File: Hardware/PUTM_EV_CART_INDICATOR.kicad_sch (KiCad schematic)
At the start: 11 parts, among them J3 Screw_Terminal_01x06

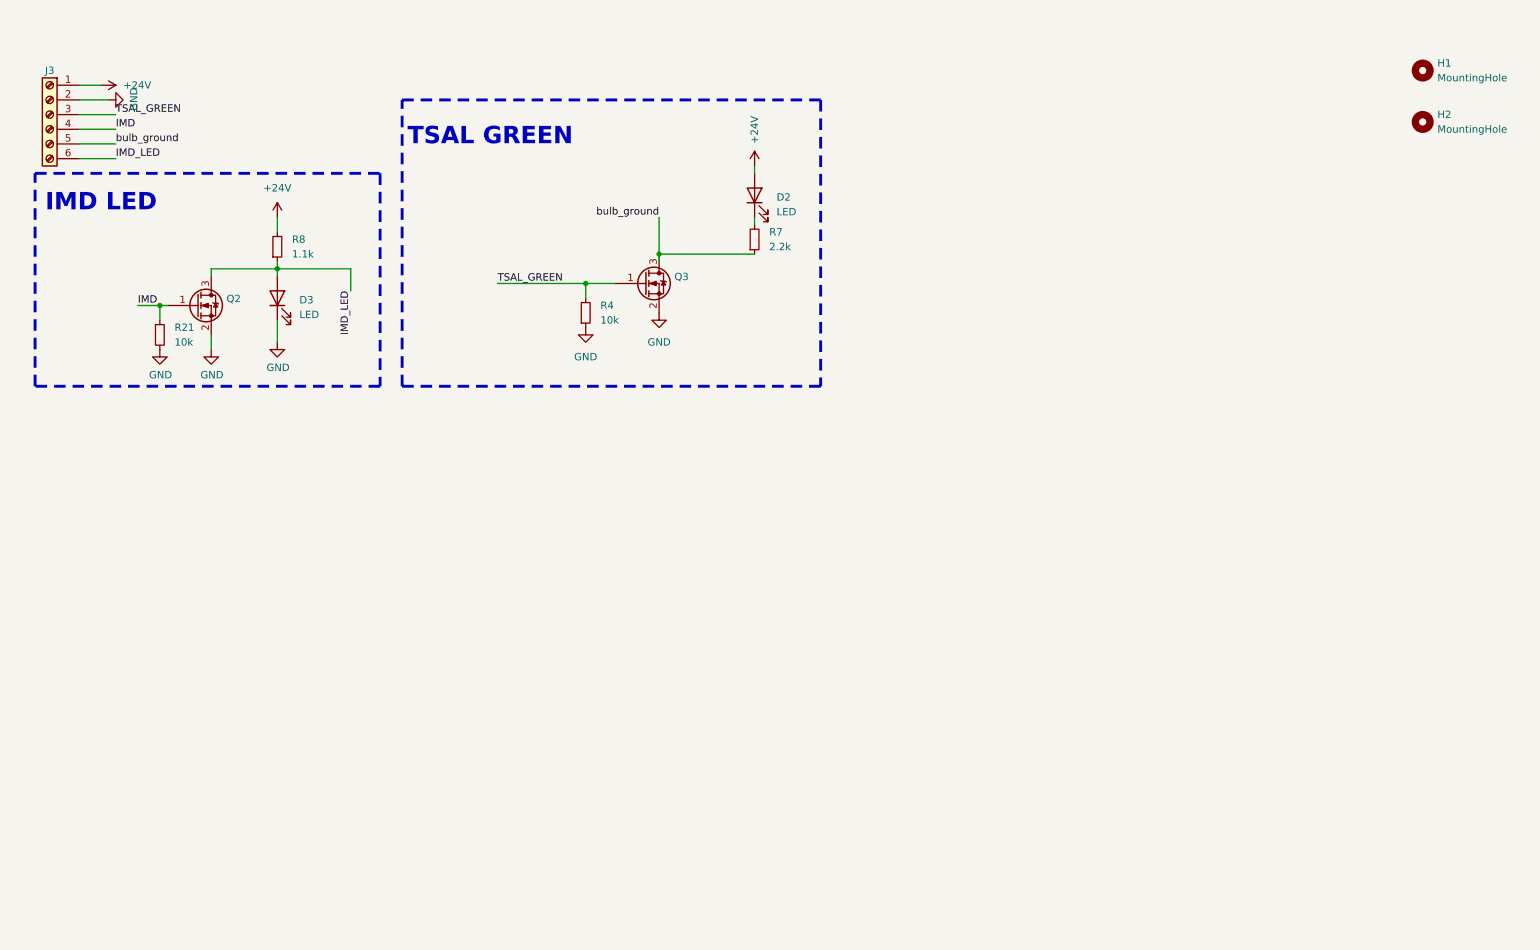
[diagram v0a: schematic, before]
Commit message: poprawy
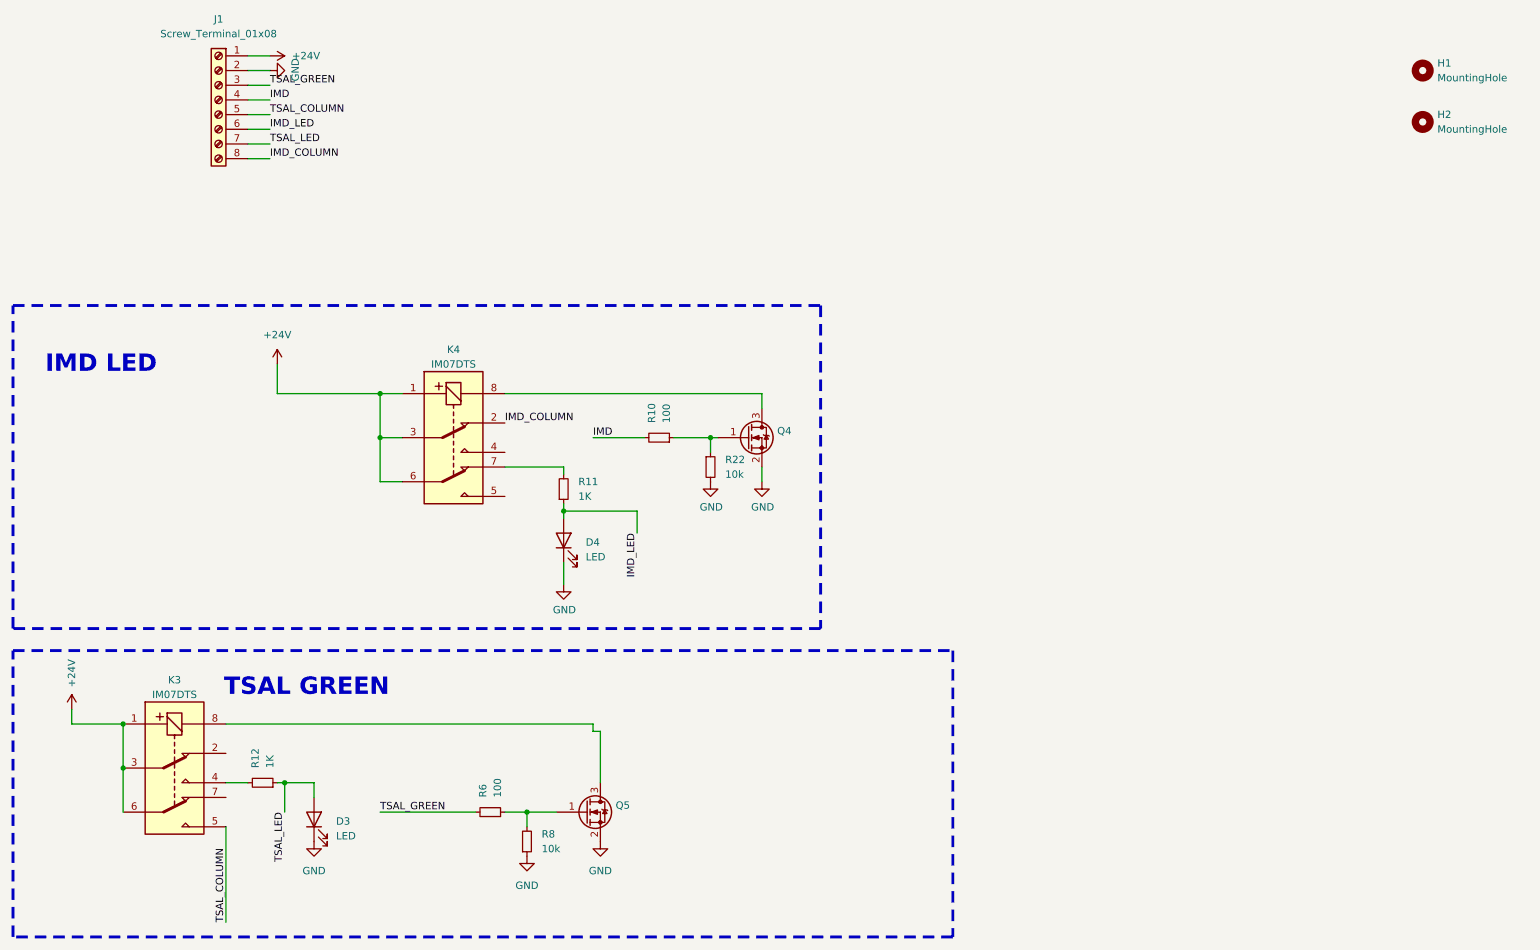
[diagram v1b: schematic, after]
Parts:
- removed D2: LED, LED_SMD:LED_0603_1608Metric, symbol Device:LED
- removed J3: Screw_Terminal_01x06, Include:TB00250006BE, symbol Connector:Screw_Terminal_01x06
- removed Q2, Q3: ~, Package_TO_SOT_SMD:SOT-23, symbol PUTM_EV_IMD_SAFETY_2021-rescue:2N7002-Transistor_FET
- removed R21, R4: 10k, Resistor_SMD:R_0603_1608Metric_Pad0.98x0.95mm_HandSolder, symbol Device:R_Small
- removed R7: 2.2k, Resistor_SMD:R_0603_1608Metric_Pad0.98x0.95mm_HandSolder, symbol Device:R_Small
- added D4: LED, LED_SMD:LED_0603_1608Metric, symbol Device:LED
- added J1: Screw_Terminal_01x08, Include:TB00150008BE, symbol Connector:Screw_Terminal_01x08
- added K3, K4: IM07DTS, Include:IM23TS, symbol Samacsys_kicad_sym:IM07DTS
- added Q4, Q5: ~, Package_TO_SOT_SMD:SOT-23, symbol PUTM_EV_IMD_SAFETY_2021-rescue:2N7002-Transistor_FET
- added R10, R6: 100, Resistor_SMD:R_0603_1608Metric_Pad0.98x0.95mm_HandSolder, symbol Device:R_Small
- added R11, R12: 1K, Resistor_SMD:R_0603_1608Metric_Pad0.98x0.95mm_HandSolder, symbol Device:R_Small
- added R22: 10k, Resistor_SMD:R_0603_1608Metric_Pad0.98x0.95mm_HandSolder, symbol Device:R_Small
- R8: value 1.1k -> 10k
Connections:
- net +24V: now also J1.1 (Pin_1), K3.1 (COIL_1), K3.3 (COM_1), K3.6 (COM_2), K4.1 (COIL_1), K4.3 (COM_1), K4.6 (COM_2); no longer R8.2
- net GND: now also R8.1, D4.1 (K), J1.2 (Pin_2), Q4.2 (S), Q5.2 (S), R22.2
- net IMD: now also J1.4 (Pin_4), R10.2
- net IMD_LED: now also D4.2 (A), J1.6 (Pin_6), R11.1; no longer D3.2 (A), R8.1
- net TSAL_GREEN: now also J1.3 (Pin_3), R6.2
- new net: Q4.1 (G), R10.1, R22.1
- new net: K4.8 (COIL_2), Q4.3 (D)
- new net: Q5.1 (G), R6.1, R8.2
- new net: K3.8 (COIL_2), Q5.3 (D)
- new net: K4.7 (NC_2), R11.2
- new net: K3.4 (NO_1), R12.2
- new net IMD_COLUMN: J1.8 (Pin_8), K4.2 (NC_1)
- new net TSAL_COLUMN: J1.5 (Pin_5), K3.5 (NO_2)
- new net TSAL_LED: D3.2 (A), J1.7 (Pin_7), R12.1
